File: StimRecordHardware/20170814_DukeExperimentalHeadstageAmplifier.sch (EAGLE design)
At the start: 1 part

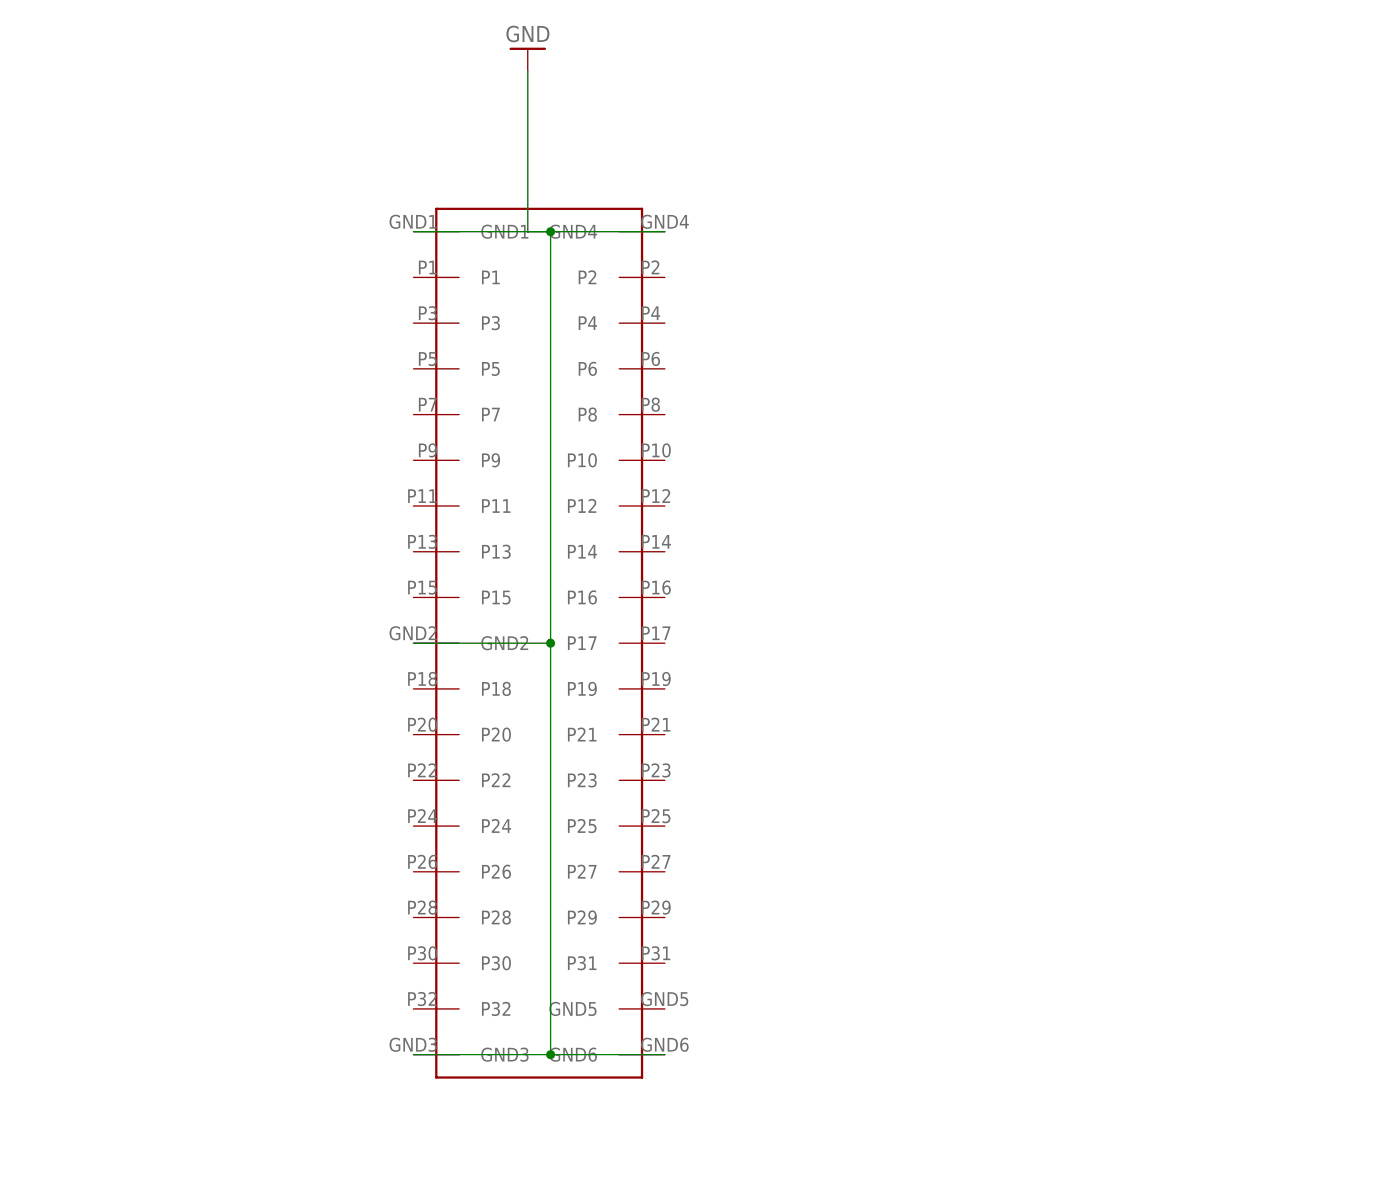
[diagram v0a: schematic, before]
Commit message: minor changes
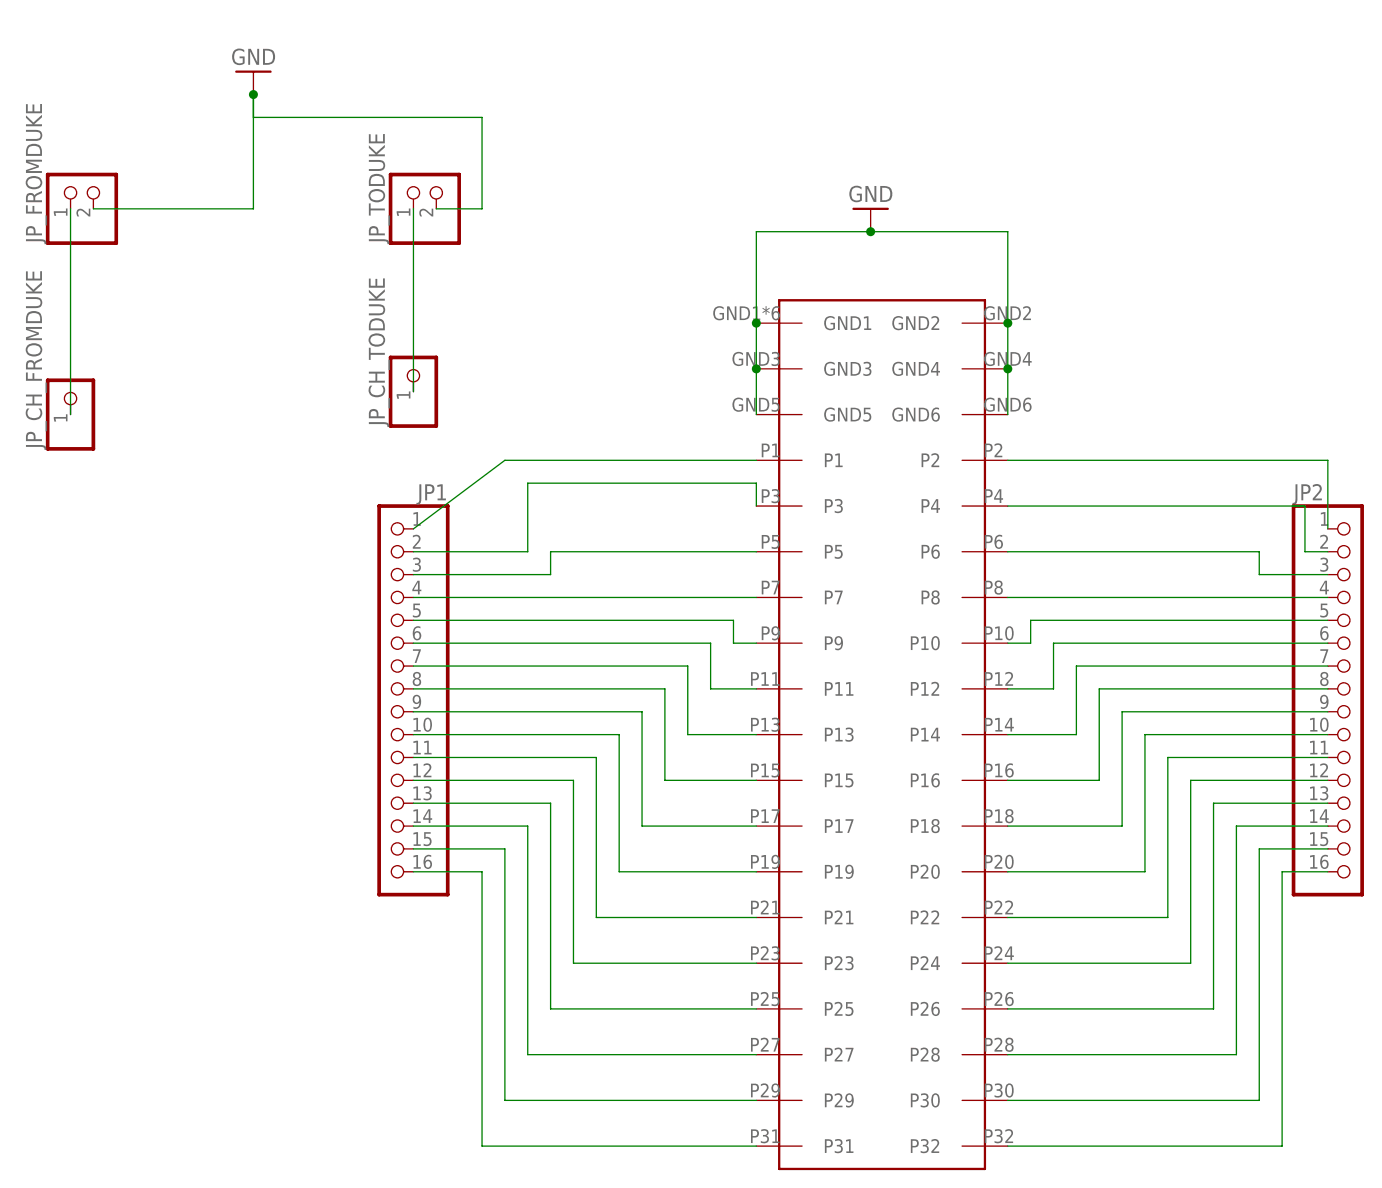
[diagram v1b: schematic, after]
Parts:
- added JP1, JP2: (no value), pinhead:PINHD-1X16
- added JP_CH_FROMDUKE, JP_CH_TODUKE: (no value), pinhead:PINHD-1X1
- added JP_FROMDUKE, JP_TODUKE: (no value), pinhead:PINHD-1X2
- U$1: value MIS-019-01-H-D-EM2 -> MIS-019-01-H-D; device MIS_38pin:MIS-019-01-H-D-EM2 -> Sombeck_lib:MIS-019-01-H-D
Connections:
- new net N$1: JP1.1, U$1.P1
- new net N$10: JP1.10, U$1.P19
- new net N$11: JP1.11, U$1.P21
- new net N$12: JP1.12, U$1.P23
- new net N$13: JP1.13, U$1.P25
- new net N$14: JP1.14, U$1.P27
- new net N$15: JP1.15, U$1.P29
- new net N$16: JP1.16, U$1.P31
- new net N$17: JP2.1, U$1.P2
- new net N$18: JP2.2, U$1.P4
- new net N$19: JP2.3, U$1.P6
- new net N$2: JP1.2, U$1.P3
- new net N$20: JP2.4, U$1.P8
- new net N$21: JP2.5, U$1.P10
- new net N$22: JP2.6, U$1.P12
- new net N$23: JP2.7, U$1.P14
- new net N$24: JP2.8, U$1.P16
- new net N$25: JP2.9, U$1.P18
- new net N$26: JP2.10, U$1.P20
- new net N$27: JP2.11, U$1.P22
- new net N$28: JP2.12, U$1.P24
- new net N$29: JP2.13, U$1.P26
- new net N$3: JP1.3, U$1.P5
- new net N$30: JP2.14, U$1.P28
- new net N$31: JP2.15, U$1.P30
- new net N$32: JP2.16, U$1.P32
- new net N$34: JP_CH_TODUKE.1, JP_TODUKE.1
- new net N$35: JP_CH_FROMDUKE.1, JP_FROMDUKE.1
- new net N$4: JP1.4, U$1.P7
- new net N$5: JP1.5, U$1.P9
- new net N$6: JP1.6, U$1.P11
- new net N$7: JP1.7, U$1.P13
- new net N$8: JP1.8, U$1.P15
- new net N$9: JP1.9, U$1.P17
- net GND: now also JP_FROMDUKE.2, JP_TODUKE.2, U$1.GND5
